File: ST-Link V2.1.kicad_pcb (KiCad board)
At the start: 2 copper layers, 32.1 x 21 mm, 43 parts, among them J1 USB_OTG, J2 Conn_01x06, J3 Conn_01x08, J4 Conn_01x08, Q1 MMBT3904, U1 USBLC6-2SC6, U2 stm32, U3 MIC5219-3.3, X1 8MHz

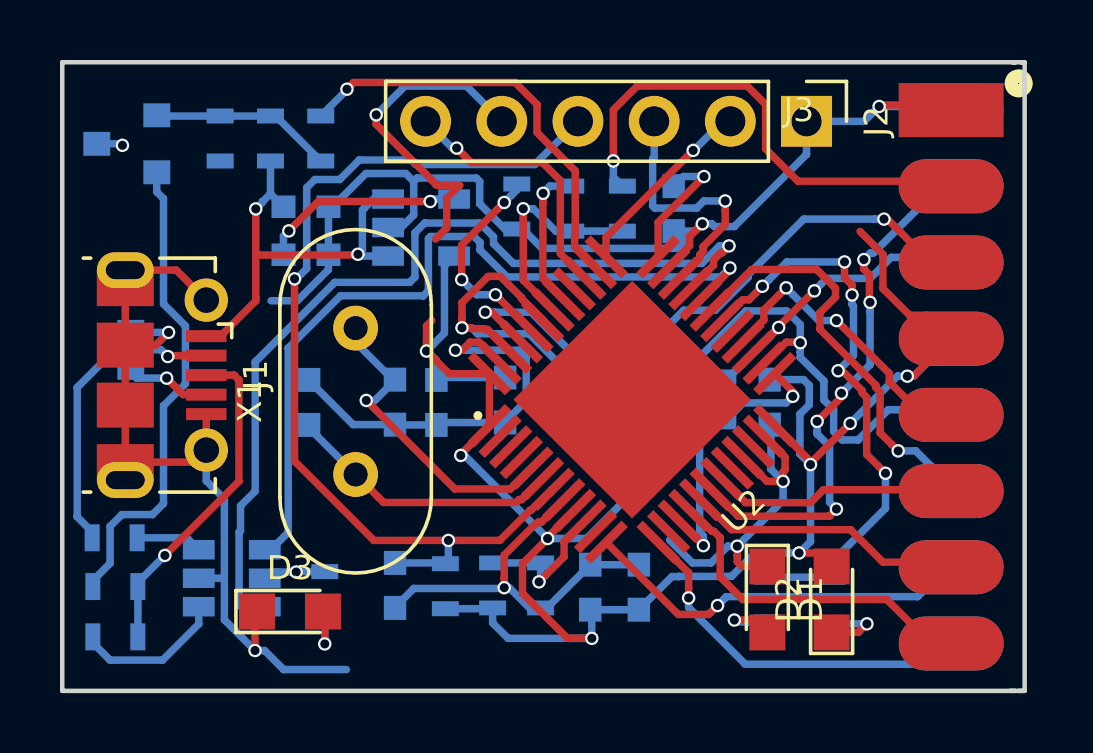
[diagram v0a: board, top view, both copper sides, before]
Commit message: minor changes
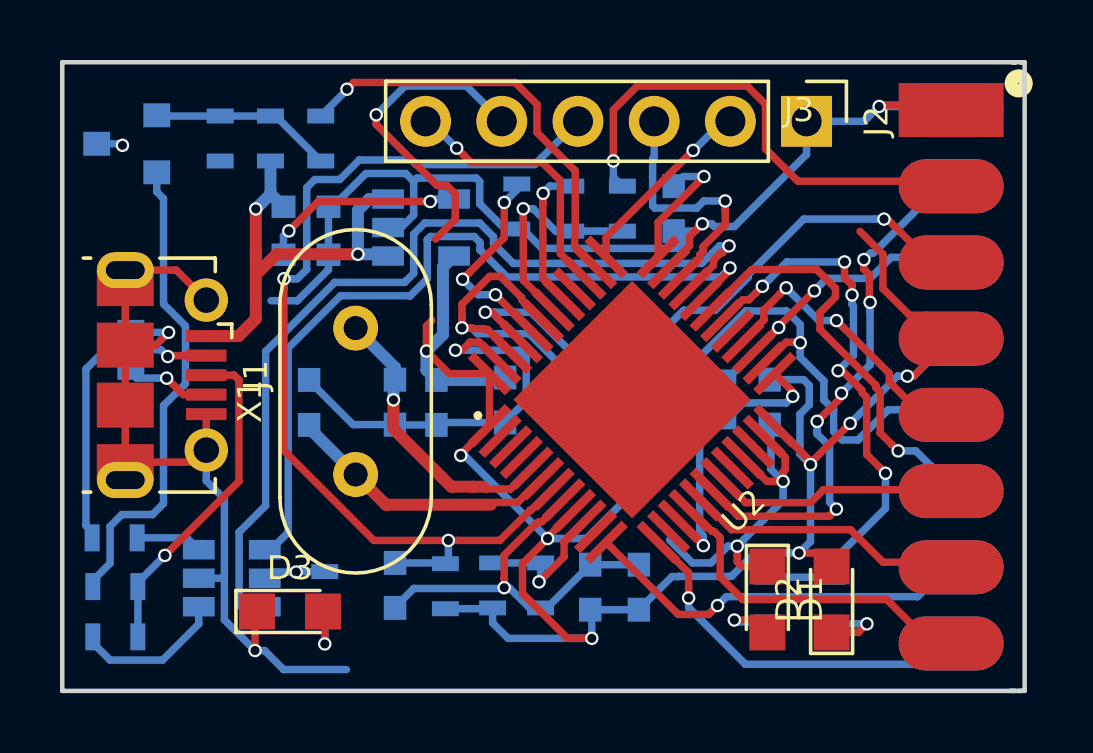
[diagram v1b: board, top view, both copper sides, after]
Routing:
- net +5V: track 15.1 -> 16.3 mm
- net Net-(C3-Pad2): track 10.6 -> 9.66 mm
- net /NRST: track 32.3 -> 32.8 mm
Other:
- net class new added: clearance 0.199999, trace_width 0.4, via_dia 0.45, via_drill 0.3
